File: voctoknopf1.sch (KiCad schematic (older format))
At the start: 46 parts, among them J1 Conn_01x02, SW1 MX_D, SW10 MX_D, SW11 MX_D, SW12 MX_D, SW2 MX_D, SW3 MX_D, SW4 MX_D, SW5 MX_D, SW6 MX_D, SW7 MX_D, SW8 MX_D, SW9 MX_D, U1 MCP23017, U2 MCP23017

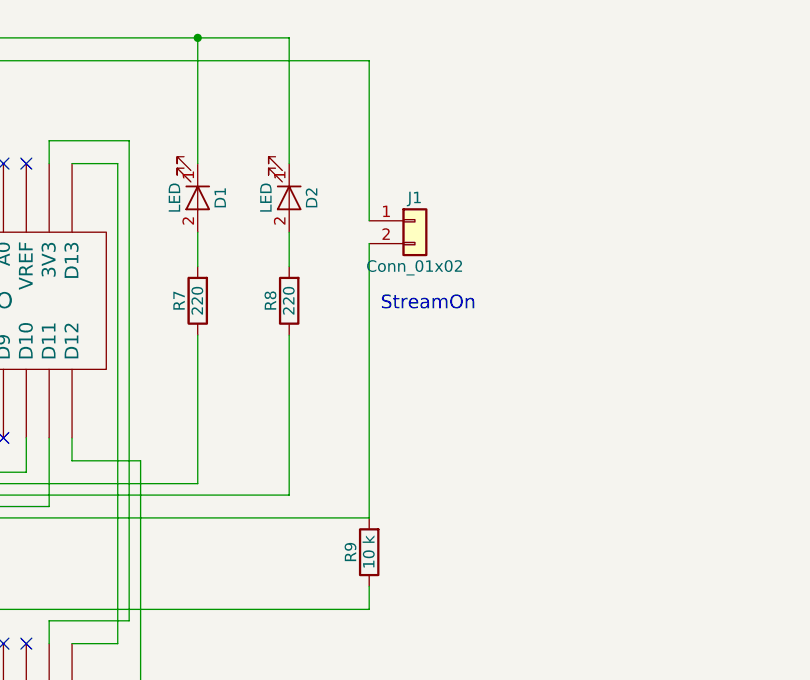
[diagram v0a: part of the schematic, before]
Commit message: netlist
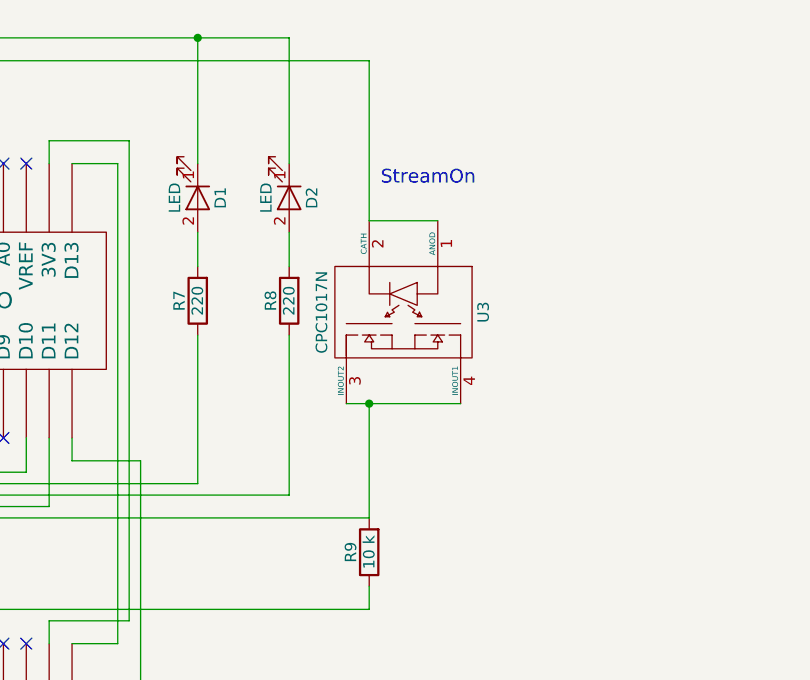
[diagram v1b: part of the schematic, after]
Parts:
- removed J1: Conn_01x02, symbol Conn_01x02
- added U3: CPC1017N, Buttons_Switches_SMD:SW_DIP_x2_W8.61mm_Slide_LowProfile, symbol CPC1017N
- D1, D2: footprint (none) -> LEDs:LED_D5.0mm
- R1, R10, R11, R12, R13, R14, R15, R16, R17, R18, R19, R2, R20, R21, R22, R23, R24, R25, R26, R27, R3, R4, R5, R6, R7, R8, R9: footprint (none) -> Resistors_THT:R_Axial_DIN0207_L6.3mm_D2.5mm_P7.62mm_Horizontal
- SW1, SW10, SW11, SW12, SW2, SW3, SW4, SW5, SW6, SW7, SW8, SW9: footprint (none) -> cherry:SW_PCB_4PIN
- U1, U2: footprint (none) -> Housings_DIP:DIP-28_W7.62mm_LongPads
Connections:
- net 5V: now also U3.1 (ANOD), U3.2 (CATH)
- net at ARDUINO1.8 (D5), R9.2: now also U3.3 (INOUT2), U3.4 (INOUT1)
